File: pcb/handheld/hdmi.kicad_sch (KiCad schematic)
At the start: 22 parts, among them J3 HDMI_A, Q3 AO3400A

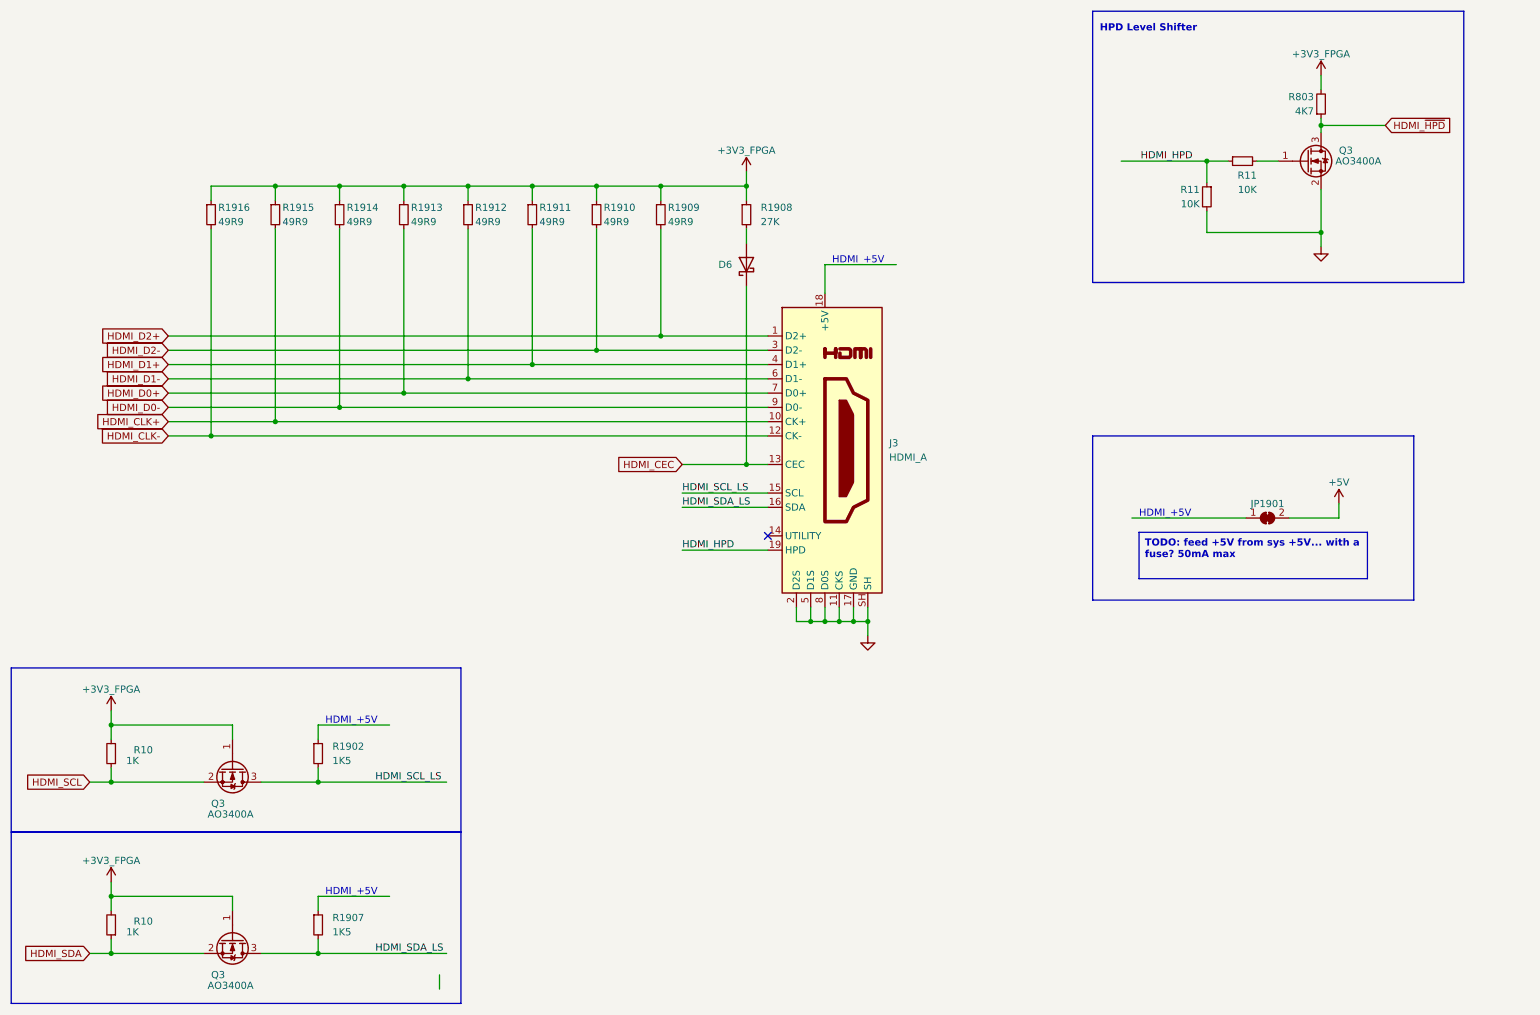
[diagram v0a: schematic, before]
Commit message: Rev A of PCB
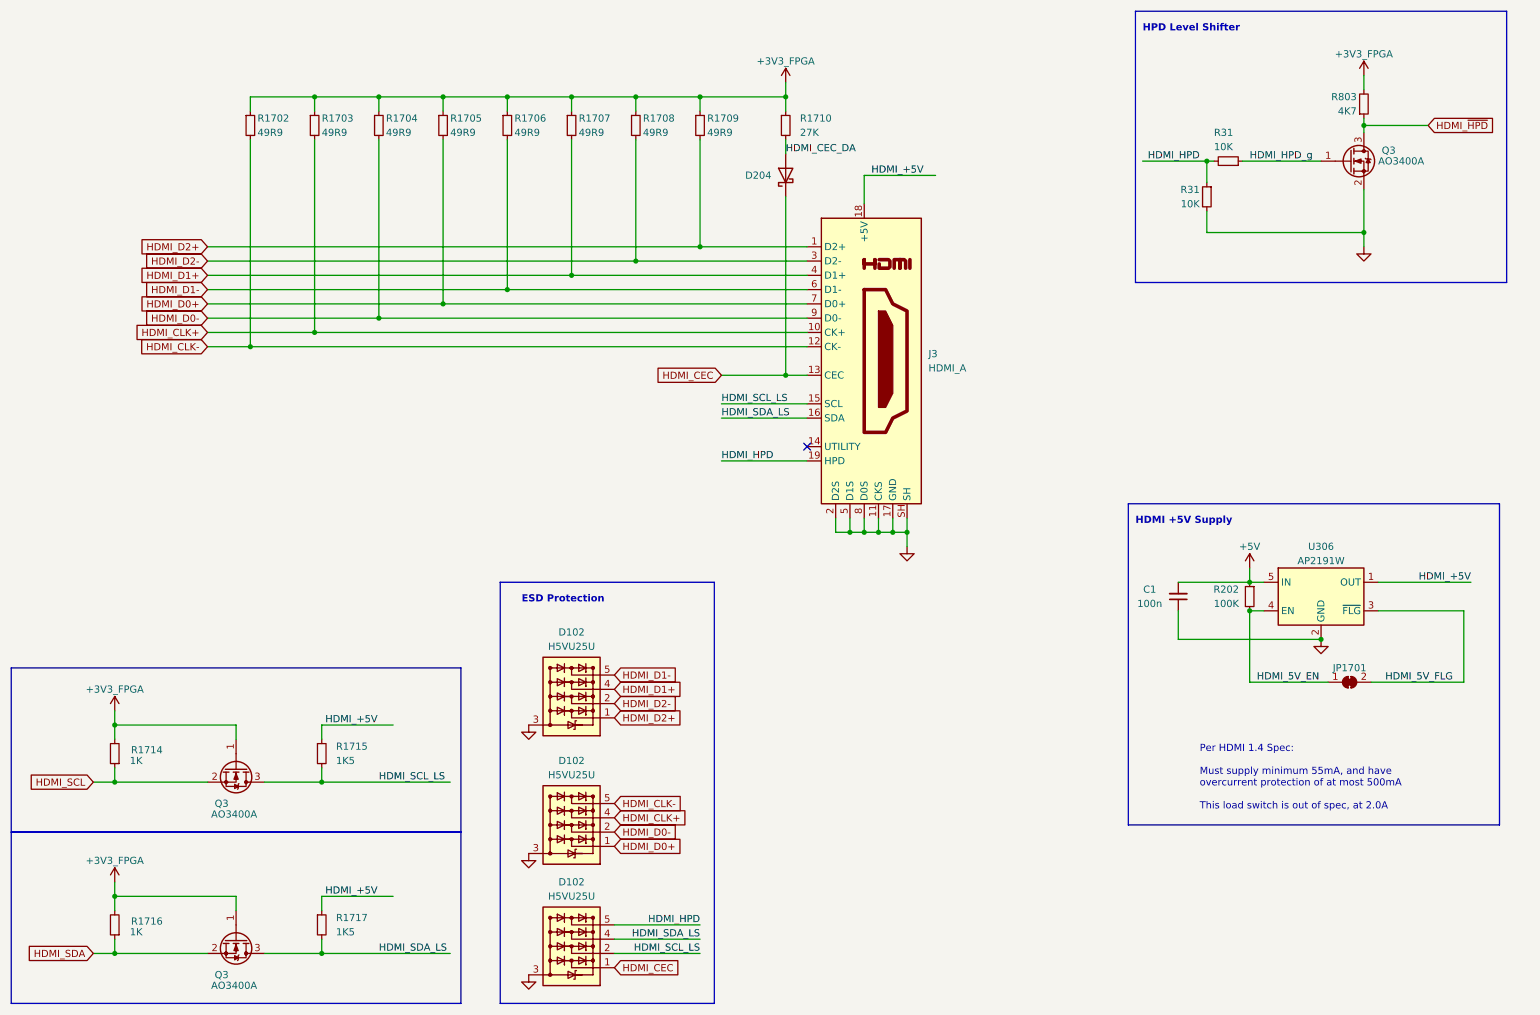
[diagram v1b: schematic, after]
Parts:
- added C1: 100n, Capacitor_SMD:C_0402_1005Metric, symbol Device:C_Small
- added D102 (x3): H5VU25U, Package_DFN_QFN:Diodes_UDFN-10_1.0x2.5mm_P0.5mm, symbol Game_Bub:H5VU25U
- added R202: 100K, Resistor_SMD:R_0402_1005Metric, symbol Device:R_Small
- added U306: AP2191W, Package_TO_SOT_SMD:SOT-23-5, symbol Game_Bub:AP2191W
- J3: footprint (none) -> Connector_HDMI:HDMI_A_Molex_208658-1001_Horizontal
- renumbered D6 to D204, JP1901 to JP1701, R1916 to R1702, R1915 to R1703, R1914 to R1704, R1913 to R1705, R1912 to R1706, R1911 to R1707, R1910 to R1708, R1909 to R1709, R1908 to R1710, R10 to R1714, R1902 to R1715, R10 to R1716, R1907 to R1717, R11 to R31
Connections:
- net +5V: now also C1.2, R202.1, U306.5 (IN); no longer JP1701.2 (B)
- net GND: now also C1.1, D102.3 (A), D102.3 (A), D102.3 (A), D102.8 (A), D102.8 (A), D102.8 (A), U306.2 (GND)
- net HDMI_CEC: now also D102.1 (K1), D102.10 (K1)
- net HDMI_CLK+: now also D102.4 (K3), D102.7 (K3)
- net HDMI_CLK-: now also D102.5 (K4), D102.6 (K4)
- net HDMI_D0+: now also D102.1 (K1), D102.10 (K1)
- net HDMI_D0-: now also D102.2 (K2), D102.9 (K2)
- net HDMI_D1+: now also D102.4 (K3), D102.7 (K3)
- net HDMI_D1-: now also D102.5 (K4), D102.6 (K4)
- net HDMI_D2+: now also D102.1 (K1), D102.10 (K1)
- net HDMI_D2-: now also D102.2 (K2), D102.9 (K2)
- net HDMI_HPD: now also R31.2, D102.5 (K4), D102.6 (K4); no longer R31.1
- net HDMI_SCL_LS: now also D102.2 (K2), D102.9 (K2)
- net HDMI_SDA_LS: now also D102.4 (K3), D102.7 (K3)
- net HDMI_CEC_DA: now reaches D204.2 (A), R1710.2
- net HDMI_5V_EN: now reaches JP1701.1 (A)
- net HDMI_5V_EN: now also R202.2, U306.4 (EN)
- net HDMI_+5V: now reaches R1717.1
- net HDMI_+5V: now also J3.18 (+5V), R1715.1, U306.1 (OUT)
- net HDMI_HPD_g: now reaches Q3.1 (G)
- net HDMI_HPD_g: now also R31.1; no longer R31.2
- new net HDMI_5V_FLG: JP1701.2 (B), U306.3 (~{FLG})
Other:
- note added: "ESD Protection"
- note added: "HDMI +5V Supply"
- note added: "Per HDMI 1.4 Spec: Must supply minimum 55mA, and have overcurrent protection of at most 500mA This load switch is out of spec, at 2.0A"
- note removed: "HDMI_+5V"
- moved on the sheet: D204, J3, JP1701, Q3, R1702, R1703, R1704, R1705, R1706, R1707, R1708, R1709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
